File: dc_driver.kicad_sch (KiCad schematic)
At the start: 30 parts, among them U2 L298N, U3 L298N, U4 L298N

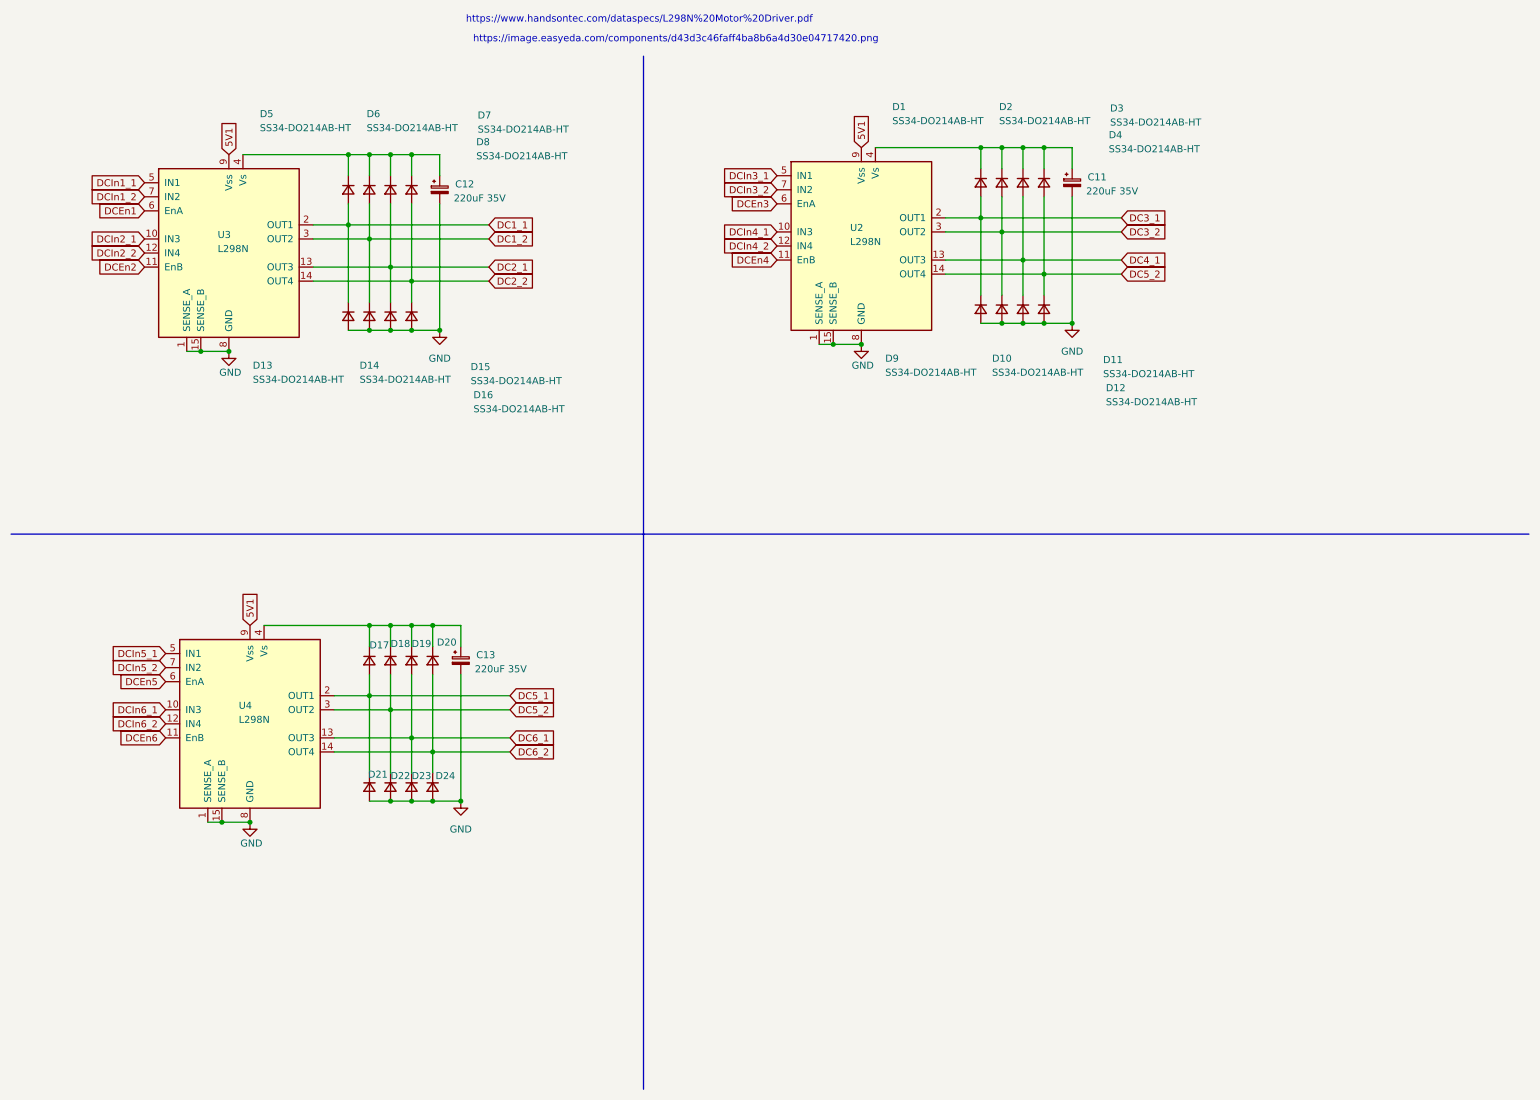
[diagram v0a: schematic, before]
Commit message: Visual Improvements
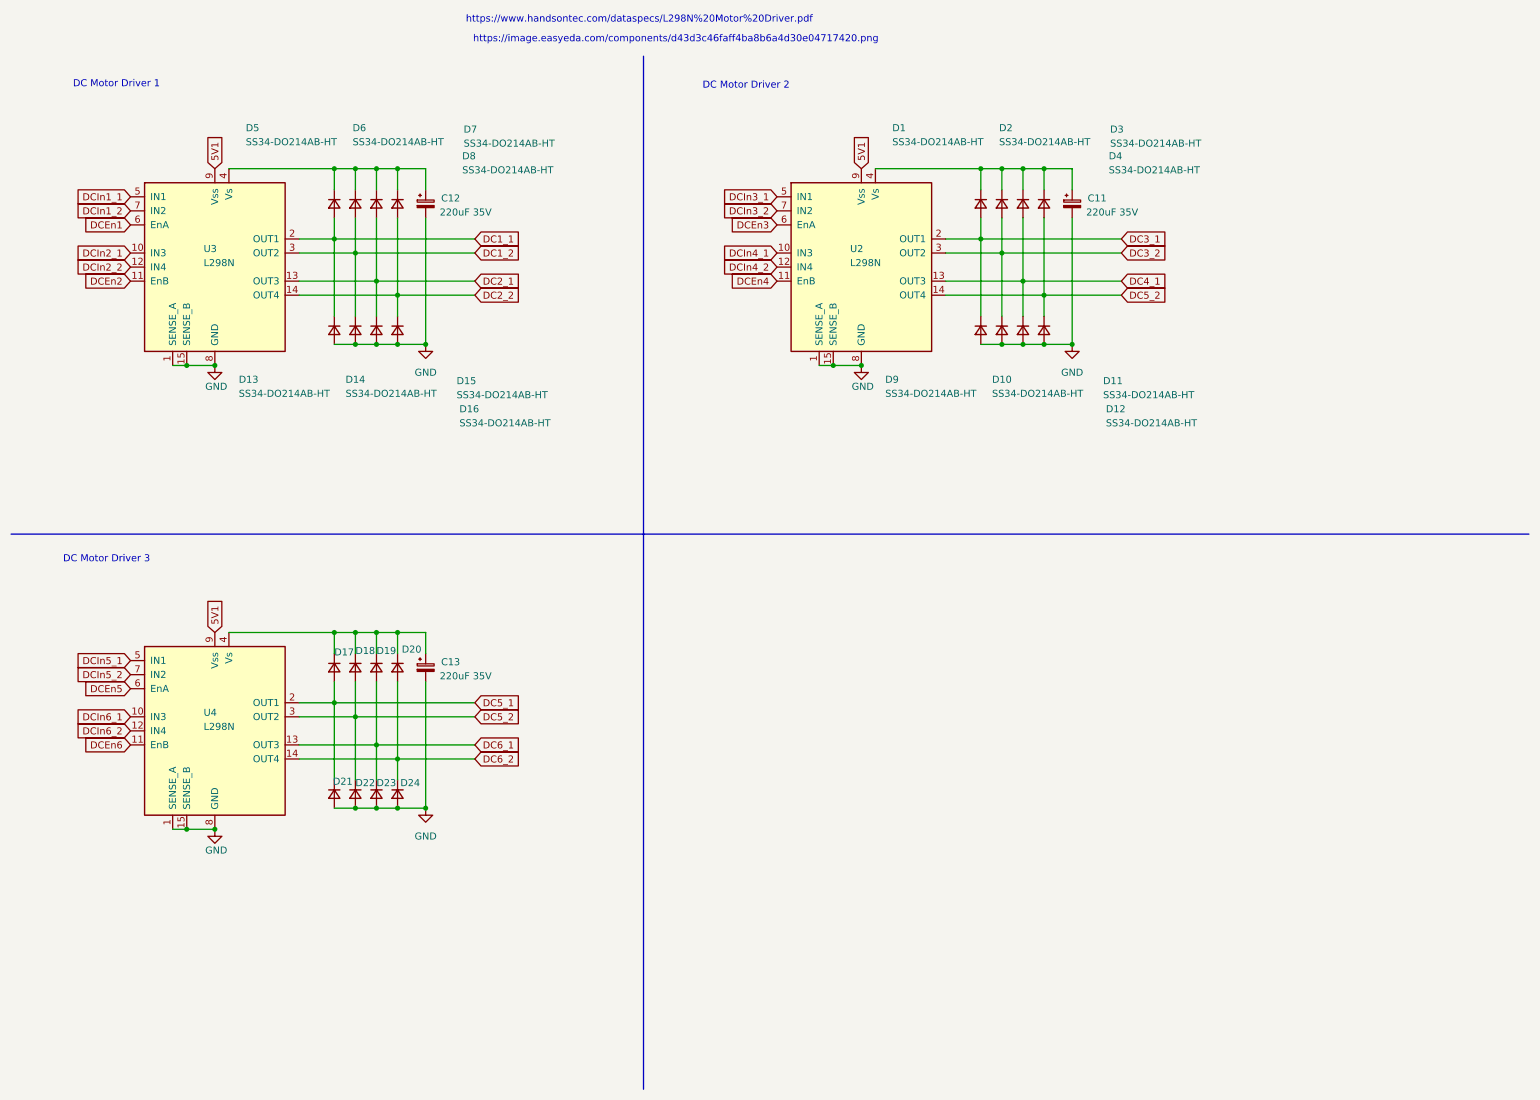
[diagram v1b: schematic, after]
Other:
- note added: "DC Motor Driver 1"
- note added: "DC Motor Driver 2"
- note added: "DC Motor Driver 3"
- moved on the sheet: C11, C12, C13, D1, D10, D11, D12, D13, D14, D15, D16, D17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
